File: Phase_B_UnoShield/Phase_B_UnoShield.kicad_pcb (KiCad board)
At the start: 2 copper layers, 98.4 x 83.8 mm, 51 parts, among them J1 USB_B_Mini, J3 AVR-ISP-6, J4 ESP_Conn, U1 CA56-12EWA, U2 74HC595, U3 ATmega32U4-A, U4 USBLC6-2SC6, U5 LP2985-3.3, Y1 16MHz

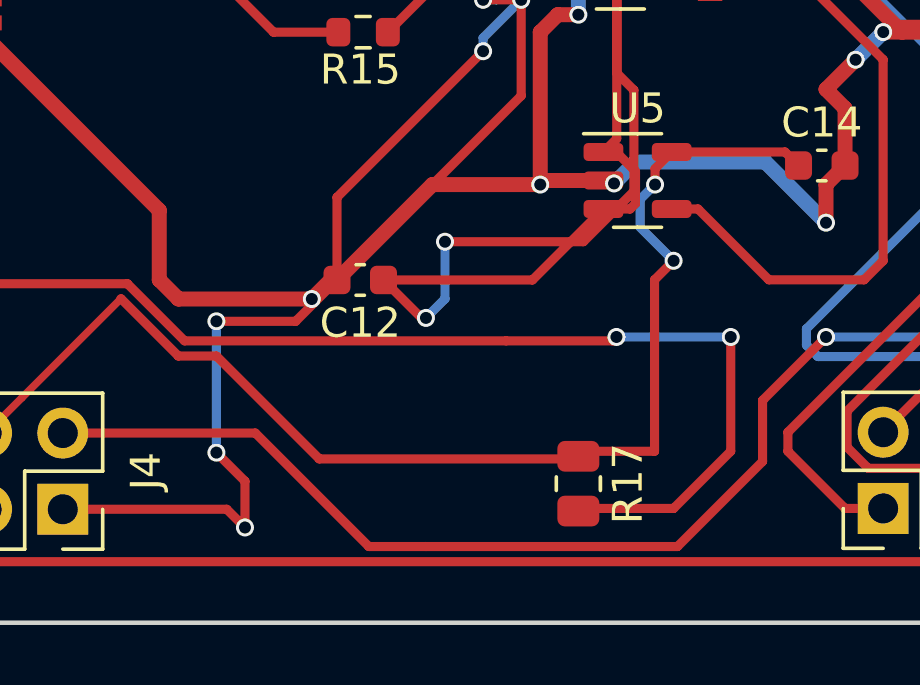
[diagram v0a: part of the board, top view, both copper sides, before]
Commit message: Edit version 2
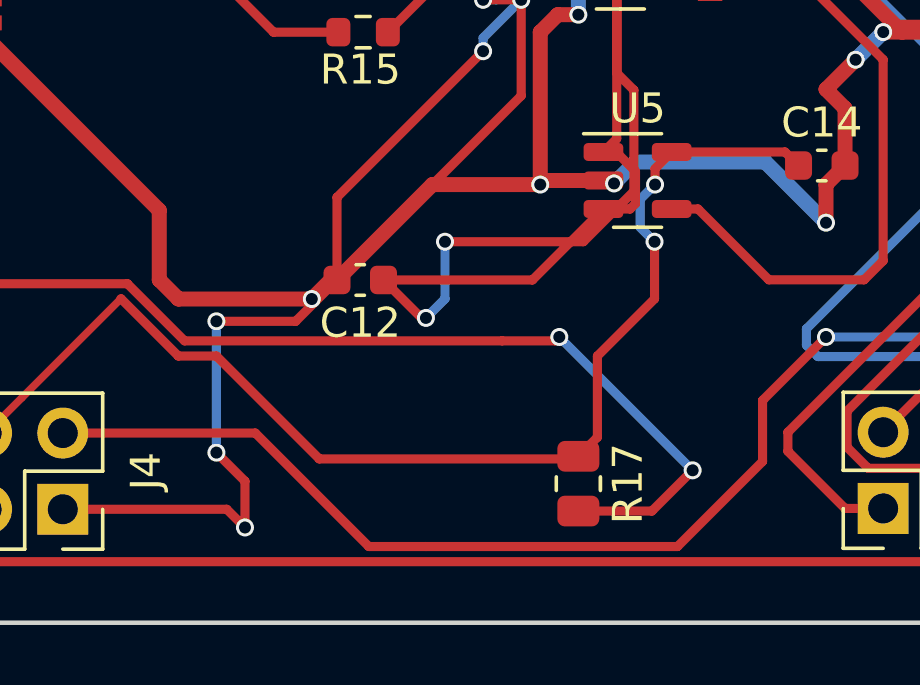
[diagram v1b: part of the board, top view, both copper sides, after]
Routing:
- net Net-(J4-Pin_5): track 49.0 -> 44.3 mm
- net +3.3V: track 47.0 -> 45.1 mm
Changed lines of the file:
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@@
   (segment (start 33.02 116.84) (end 31.115 114.935) (width 0.305) (layer "F.Cu") (net 44))
   (segment (start 53.244174 110.039174) (end 53.695 110.49) (width 0.305) (layer "F.Cu") (net 44))
-  (segment (start 48.895 114.3) (end 48.895 120.015) (width 0.305) (layer "F.Cu") (net 44))
   (segment (start 26.629549 119.407651) (end 27.804549 118.232651) (width 0.25) (layer "F.Cu") (net 44))
   (segment (start 24.089549 119.407651) (end 26.629549 119.407651) (width 0.305) (layer "F.Cu") (net 44))
   (segment (start 48.912 111.125) (end 48.912 110.593886) (width 0.305) (layer "F.Cu") (net 44))
   (segment (start 21.549549 119.407651) (end 24.089549 119.407651) (width 0.305) (layer "F.Cu") (net 44))
+  (segment (start 48.895 114.935) (end 46.99 116.84) (width 0.305) (layer "F.Cu") (net 44))
   (segment (start 31.115 114.935) (end 31.1022 114.935) (width 0.305) (layer "F.Cu") (net 44))
   (segment (start 37.72 120.27) (end 34.29 116.84) (width 0.305) (layer "F.Cu") (net 44))
+  (segment (start 46.99 116.84) (end 46.99 119.5475) (width 0.305) (layer "F.Cu") (net 44))
   (segment (start 48.912 110.593886) (end 49.466712 110.039174) (width 0.305) (layer "F.Cu") (net 44))
   (segment (start 46.355 120.27) (end 37.72 120.27) (width 0.305) (layer "F.Cu") (net 44))
   (segment (start 49.466712 110.039174) (end 53.244174 110.039174) (width 0.305) (layer "F.Cu") (net 44))
-  (segment (start 49.53 113.665) (end 48.895 114.3) (width 0.305) (layer "F.Cu") (net 44))
-  (segment (start 46.5225 120.015) (end 46.355 120.1825) (width 0.305) (layer "F.Cu") (net 44))
+  (segment (start 48.895 113.03) (end 48.895 114.935) (width 0.305) (layer "F.Cu") (net 44))
+  (segment (start 46.99 119.5475) (end 46.355 120.1825) (width 0.305) (layer "F.Cu") (net 44))
   (segment (start 27.804549 118.232651) (end 31.1022 114.935) (width 0.25) (layer "F.Cu") (net 44))
-  (segment (start 48.895 120.015) (end 46.5225 120.015) (width 0.305) (layer "F.Cu") (net 44))
   (segment (start 34.29 116.84) (end 33.02 116.84) (width 0.305) (layer "F.Cu") (net 44))
-  (via (at 49.53 113.665) (size 0.6) (drill 0.4) (layers "F.Cu" "B.Cu") (net 44))
+  (via (at 48.895 113.03) (size 0.6) (drill 0.4) (layers "F.Cu" "B.Cu") (net 44))
   (via (at 48.912 111.125) (size 0.6) (drill 0.4) (layers "F.Cu" "B.Cu") (net 44))
-  (segment (start 48.417158 112.552158) (end 49.53 113.665) (width 0.305) (layer "B.Cu") (net 44))
-  (segment (start 48.912 111.125) (end 48.417158 111.619842) (width 0.305) (layer "B.Cu") (net 44))
   (segment (start 48.417158 111.619842) (end 48.417158 112.552158) (width 0.305) (layer "B.Cu") (net 44))
+  (segment (start 48.417158 111.619842) (end 48.912 111.125) (width 0.305) (layer "B.Cu") (net 44))
+  (segment (start 48.417158 112.552158) (end 48.895 113.03) (width 0.305) (layer "B.Cu") (net 44))
   (segment (start 26.135 103.335) (end 32.555 103.335) (width 0.305) (layer "F.Cu") (net 47))
   (segment (start 35.56 100.33) (end 37.590001 100.33) (width 0.305) (layer "F.Cu") (net 47))
@@
   (via (at 54.61 116.205) (size 0.6) (drill 0.4) (layers "F.Cu" "B.Cu") (net 52))
   (segment (start 54.61 116.205) (end 67.31 116.205) (width 0.305) (layer "B.Cu") (net 52))
-  (segment (start 43.945 116.335) (end 47.495 116.335) (width 0.305) (layer "F.Cu") (net 54))
+  (segment (start 43.815 116.335) (end 45.59 116.335) (width 0.305) (layer "F.Cu") (net 54))
+  (segment (start 33.229178 116.335) (end 43.815 116.335) (width 0.305) (layer "F.Cu") (net 54))
   (segment (start 24.826608 114.43) (end 31.324178 114.43) (width 0.305) (layer "F.Cu") (net 54))
-  (segment (start 33.229178 116.335) (end 43.945 116.335) (width 0.305) (layer "F.Cu") (net 54))
-  (segment (start 47.495 116.335) (end 47.625 116.205) (width 0.305) (layer "F.Cu") (net 54))
   (segment (start 20.347049 119.905743) (end 20.347049 118.909559) (width 0.305) (layer "F.Cu") (net 54))
+  (segment (start 45.59 116.335) (end 45.72 116.205) (width 0.305) (layer "F.Cu") (net 54))
   (segment (start 24.089549 121.947651) (end 22.752049 120.610151) (width 0.305) (layer "F.Cu") (net 54))
-  (segment (start 49.53 121.92) (end 46.4425 121.92) (width 0.305) (layer "F.Cu") (net 54))
-  (segment (start 51.435 120.015) (end 49.53 121.92) (width 0.305) (layer "F.Cu") (net 54))
-  (segment (start 51.435 116.205) (end 51.435 120.015) (width 0.305) (layer "F.Cu") (net 54))
+  (segment (start 48.8075 122.0075) (end 46.355 122.0075) (width 0.305) (layer "F.Cu") (net 54))
+  (segment (start 50.165 120.65) (end 48.8075 122.0075) (width 0.305) (layer "F.Cu") (net 54))
   (segment (start 20.347049 118.909559) (end 24.826608 114.43) (width 0.305) (layer "F.Cu") (net 54))
   (segment (start 31.324178 114.43) (end 33.229178 116.335) (width 0.305) (layer "F.Cu") (net 54))
   (segment (start 21.051457 120.610151) (end 20.347049 119.905743) (width 0.305) (layer "F.Cu") (net 54))
   (segment (start 22.752049 120.610151) (end 21.051457 120.610151) (width 0.305) (layer "F.Cu") (net 54))
-  (via (at 51.435 116.205) (size 0.6) (drill 0.4) (layers "F.Cu" "B.Cu") (net 54))
-  (via (at 47.625 116.205) (size 0.6) (drill 0.4) (layers "F.Cu" "B.Cu") (net 54))
-  (segment (start 47.625 116.205) (end 51.435 116.205) (width 0.305) (layer "B.Cu") (net 54))
+  (via (at 45.72 116.205) (size 0.6) (drill 0.4) (layers "F.Cu" "B.Cu") (net 54))
+  (via (at 50.165 120.65) (size 0.6) (drill 0.4) (layers "F.Cu" "B.Cu") (net 54))
+  (segment (start 45.72 116.205) (end 50.165 120.65) (width 0.305) (layer "B.Cu") (net 54))
   (segment (start 21.549549 121.947651) (end 23.296898 123.695) (width 0.305) (layer "F.Cu") (net 56))
   (segment (start 68.58 114.935) (end 68.605 114.91) (width 0.305) (layer "F.Cu") (net 56))
